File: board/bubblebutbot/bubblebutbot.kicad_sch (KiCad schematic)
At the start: 23 parts, among them J1 Screw_Terminal_01x02, J2 Screw_Terminal_01x02, J3 Conn_01x06_Female, J4 Conn_01x06_Female, J5 Screw_Terminal_01x02, J6 Screw_Terminal_01x02, Q1 FDN336P, U1 WeMos_D1_mini, U3 TPS613222ADBV

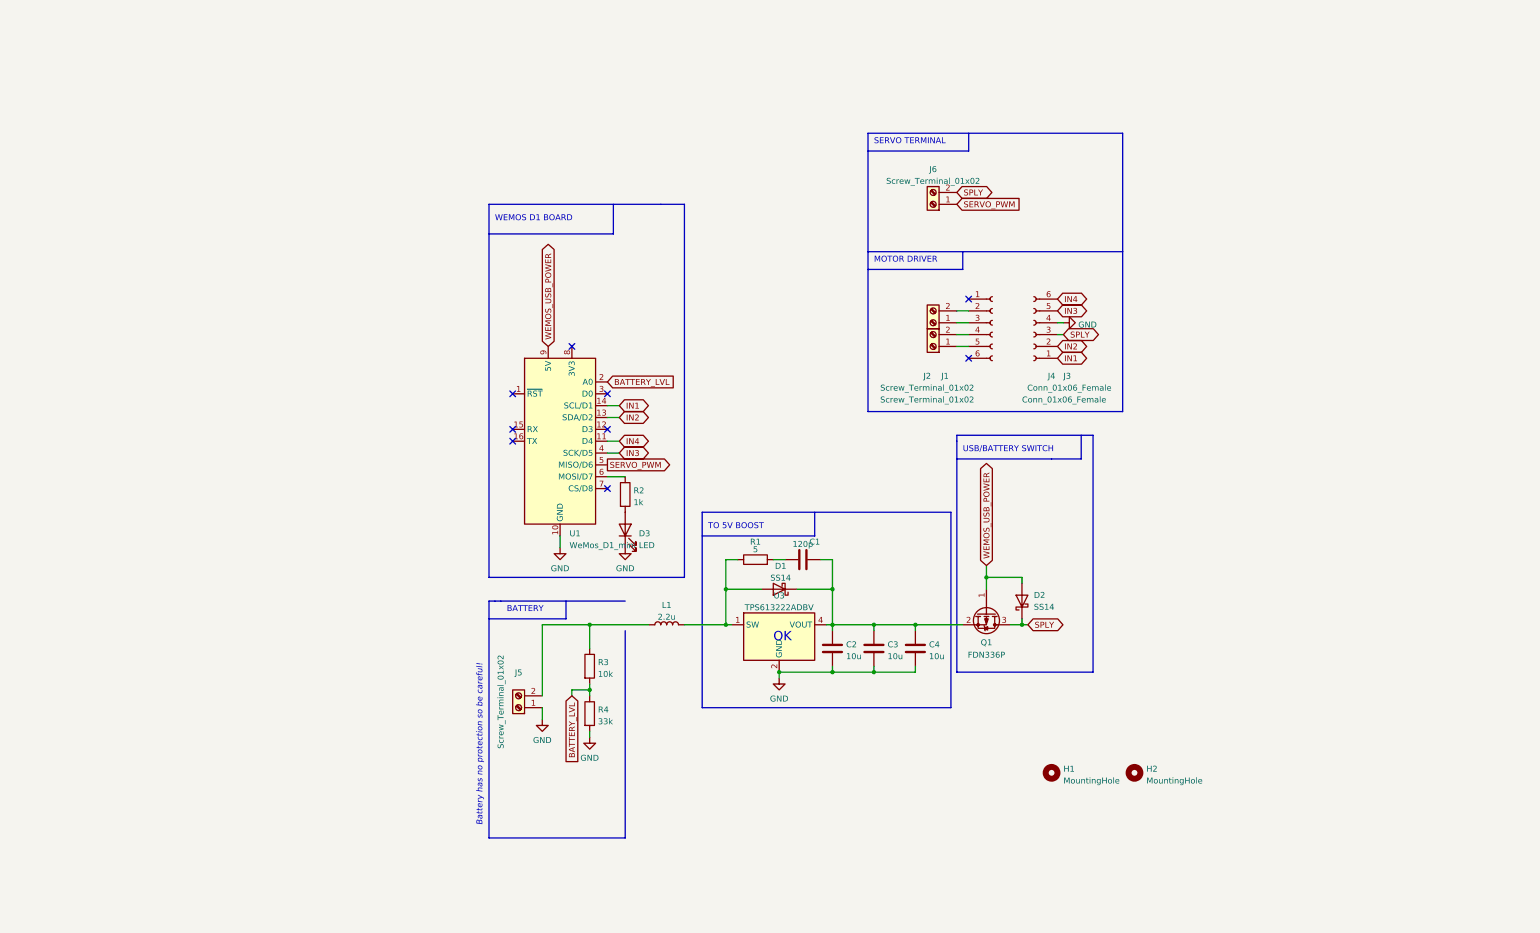
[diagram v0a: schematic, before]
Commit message: gerber for 1v01 ready
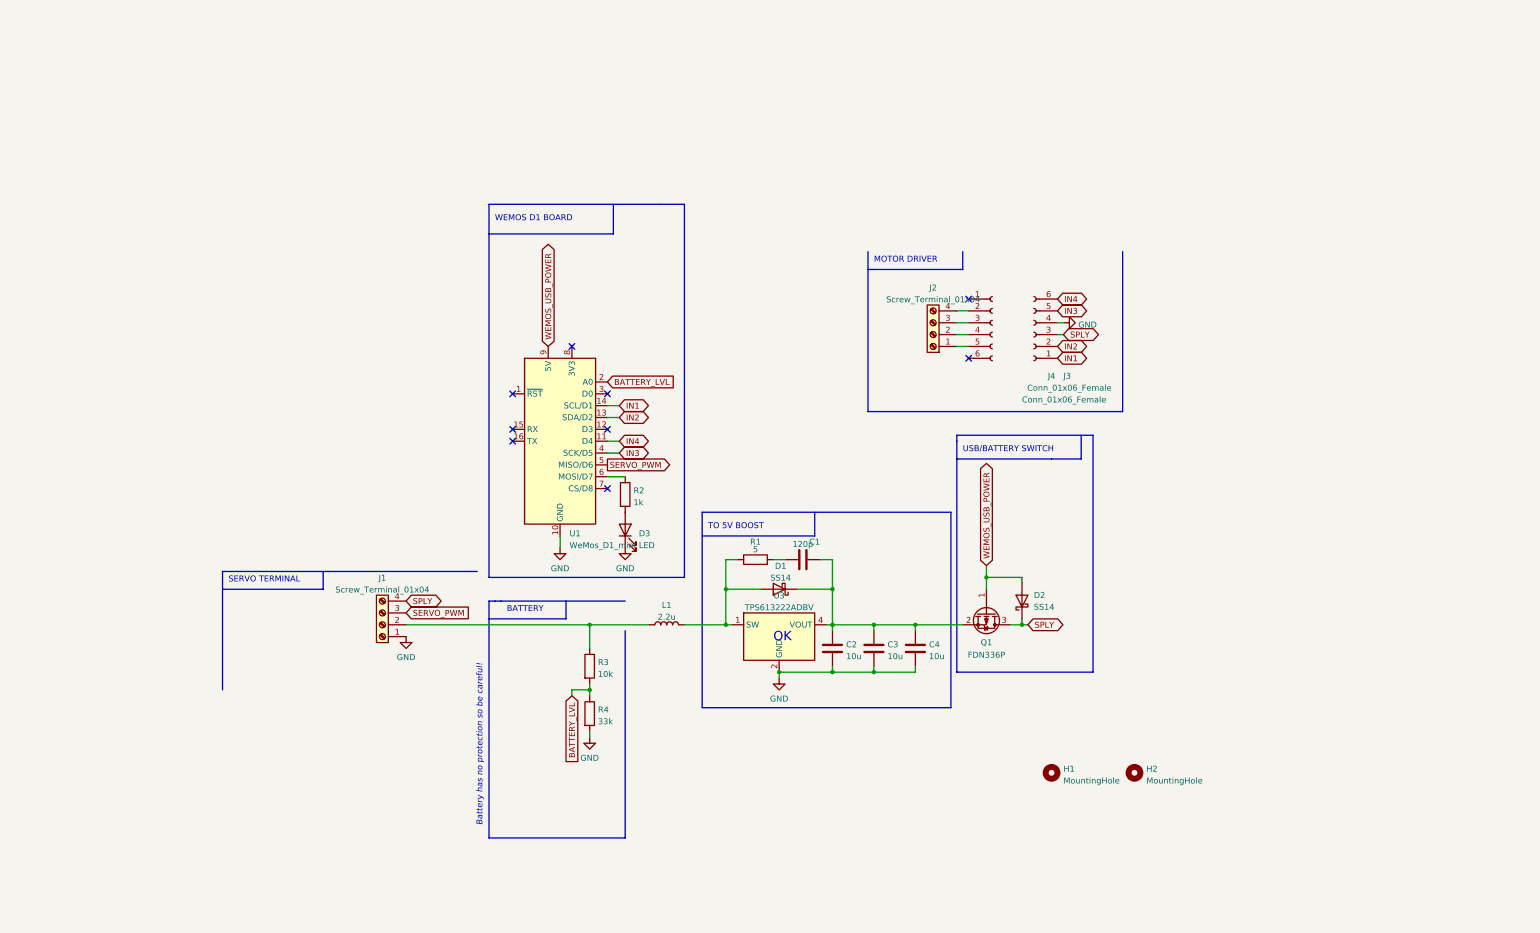
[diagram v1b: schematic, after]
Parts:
- removed J1, J2, J5, J6: Screw_Terminal_01x02, TerminalBlock:TerminalBlock_bornier-2_P5.08mm, symbol Connector:Screw_Terminal_01x02
- added J1, J2: Screw_Terminal_01x04, TerminalBlock_MetzConnect:TerminalBlock_MetzConnect_Type094_RT03504HBLU_1x04_P5.00mm_Horizontal, symbol Connector:Screw_Terminal_01x04
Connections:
- net GND: now also J1.1 (Pin_1)
- net SERVO_PWM: now also J1.3 (Pin_3)
- net SPLY: now also J1.4 (Pin_4)
- net at L1.1, R3.1: now also J1.2 (Pin_2)
- net at J3.3 (Pin_3): now also J2.3 (Pin_3)
- net at J3.2 (Pin_2): now also J2.4 (Pin_4)
- net at J3.4 (Pin_4): now also J2.2 (Pin_2)
- net at J3.5 (Pin_5): now also J2.1 (Pin_1)

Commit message: first steps into the final prod pcb!
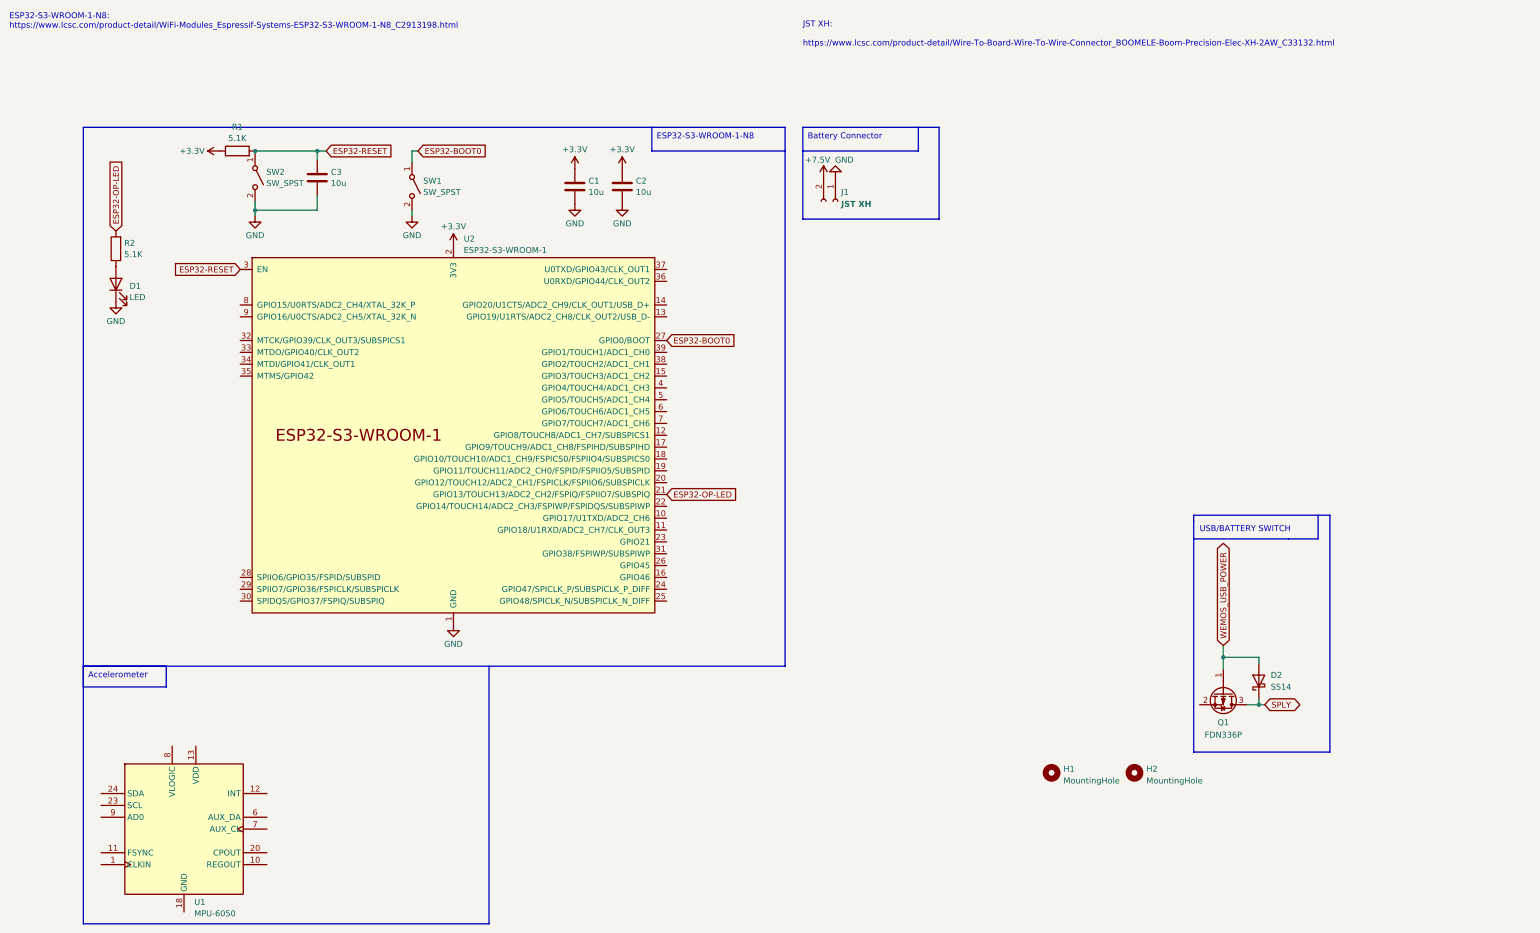
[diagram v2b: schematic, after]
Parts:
- removed C4: 10u, Capacitor_SMD:C_0603_1608Metric_Pad1.08x0.95mm_HandSolder, symbol Device:C
- removed D1: SS14, Diode_SMD:D_SMA, symbol Device:D_Schottky
- removed D3: LED, LED_SMD:LED_0603_1608Metric_Pad1.05x0.95mm_HandSolder, symbol Device:LED
- removed J1, J2: Screw_Terminal_01x04, TerminalBlock_MetzConnect:TerminalBlock_MetzConnect_Type094_RT03504HBLU_1x04_P5.00mm_Horizontal, symbol Connector:Screw_Terminal_01x04
- removed J3, J4: Conn_01x06_Female, Connector_PinSocket_2.54mm:PinSocket_1x06_P2.54mm_Vertical, symbol Connector:Conn_01x06_Female
- removed L1: 2.2u, Inductor_SMD:L_Coilcraft_LPS4018, symbol Device:L
- removed R3: 10k, Resistor_SMD:R_0603_1608Metric_Pad0.98x0.95mm_HandSolder, symbol Device:R
- removed R4: 33k, Resistor_SMD:R_0603_1608Metric_Pad0.98x0.95mm_HandSolder, symbol Device:R
- removed U1: WeMos_D1_mini, Module:WEMOS_D1_mini_light, symbol MCU_Module:WeMos_D1_mini
- removed U3: TPS613222ADBV, Package_TO_SOT_SMD:SOT-23-5, symbol Regulator_Switching:TPS613222ADBV
- added D1: LED, symbol Device:LED
- added J1: JST XH, symbol Connector:Conn_01x02_Socket
- added SW1, SW2: SW_SPST, symbol Switch:SW_SPST
- added U1: MPU-6050, Sensor_Motion:InvenSense_QFN-24_4x4mm_P0.5mm, symbol Sensor_Motion:MPU-6050
- added U2: ESP32-S3-WROOM-1, Espressif:ESP32-S3-WROOM-1, symbol PCM_Espressif:ESP32-S3-WROOM-1
- C1: value 120p -> 10u; LCSC C1643 -> C380316
- C2, C3: LCSC C19702 -> C380316
- R1: value 5 -> 5.1K; footprint Resistor_SMD:R_0805_2012Metric_Pad1.20x1.40mm_HandSolder -> (none); LCSC C17724 -> C2907114; descp 5 OHM 5% 1/3W 0805 -> (none)
- R2: value 1k -> 5.1K; footprint Resistor_SMD:R_0603_1608Metric_Pad0.98x0.95mm_HandSolder -> (none); LCSC C21190 -> C2907114
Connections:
- net GND: now also C1.2, D1.1 (K), J1.1 (Pin_1), SW1.2 (B), SW2.2 (B), U2.1 (GND), U2.40 (GND), U2.41 (GND)
- net ESP32-OP-LED: now reaches R2.2
- net ESP32-OP-LED: now also U2.21 (GPIO13/TOUCH13/ADC2_CH2/FSPIQ/FSPIIO7/SUBSPIQ)
- net +3.3V: now reaches R1.1
- net +3.3V: now also C1.1, C2.1, U2.2 (3V3)
- net ESP32-RESET: now reaches R1.2
- net ESP32-RESET: now also C3.1, SW2.1 (A), U2.3 (EN); no longer C1.1
- net at R2.1: now also D1.2 (A)
- new net +7.5V: J1.2 (Pin_2)
- new net ESP32-BOOT0: SW1.1 (A), U2.27 (GPIO0/BOOT)
- now unconnected: Q1.2 (S)
- no-connect marks 9 -> 0
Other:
- note added: "ESP32-S3-WROOM-1-N8: https://www.lcsc.com/product-detail/WiFi-Modules_Espressif-Systems-ESP32-S3-WROOM-1-N8_C2913198.html"
- note added: "JST XH: https://www.lcsc.com/product-detail/Wire-To-Board-Wire-To-Wire-Connector_BOOMELE-Boom-Precision-Elec-XH-2AW_C33132.html"
- note removed: "BATTERY"
- note removed: "Battery has no protection so be careful!"
- note removed: "MOTOR DRIVER"
- note removed: "OK"
- note removed: "SERVO TERMINAL"
- note removed: "TO 5V BOOST"
- note removed: "WEMOS D1 BOARD"
- moved on the sheet: D2, Q1
